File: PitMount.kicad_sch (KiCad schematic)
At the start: 17 parts, among them J1 Conn_01x07, Q1 BC817, Q2 IRLML6401, U1 UnifyNano, U2 ELRS-Rx

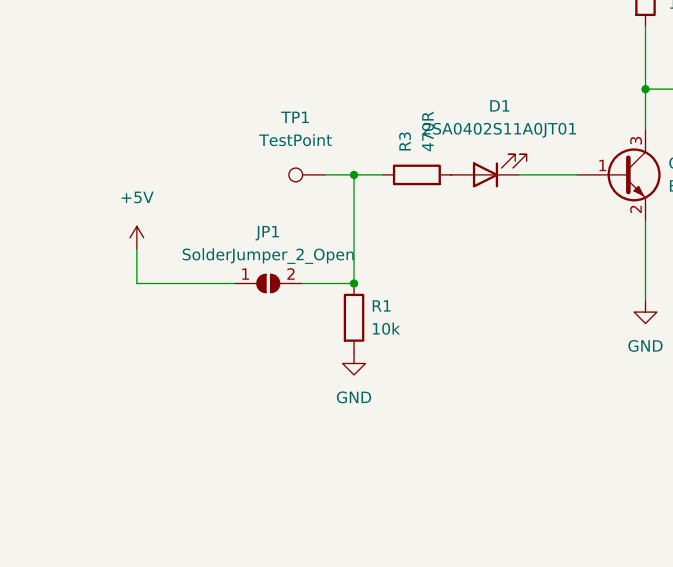
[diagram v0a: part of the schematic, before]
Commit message: Update project files with version 7.0-rc1
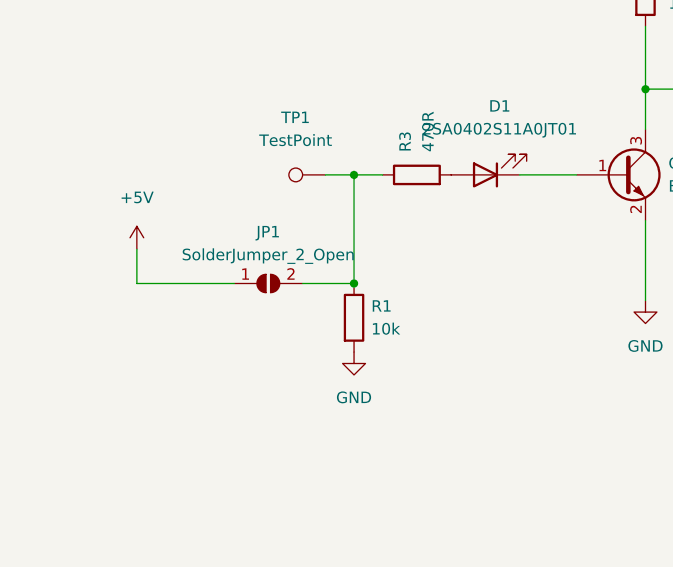
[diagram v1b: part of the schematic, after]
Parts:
- Q1, Q2: JLCPCB Rotation Offset (none) -> 180
